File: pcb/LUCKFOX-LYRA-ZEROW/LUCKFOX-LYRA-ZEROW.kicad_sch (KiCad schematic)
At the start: 4 parts, among them U1 Luckfox_Lyra_Zero_W, U2 ME54BS12-nRF54L15, U3 ME54BS01-nRF54L15, U4 MCP2518FD-xQBB

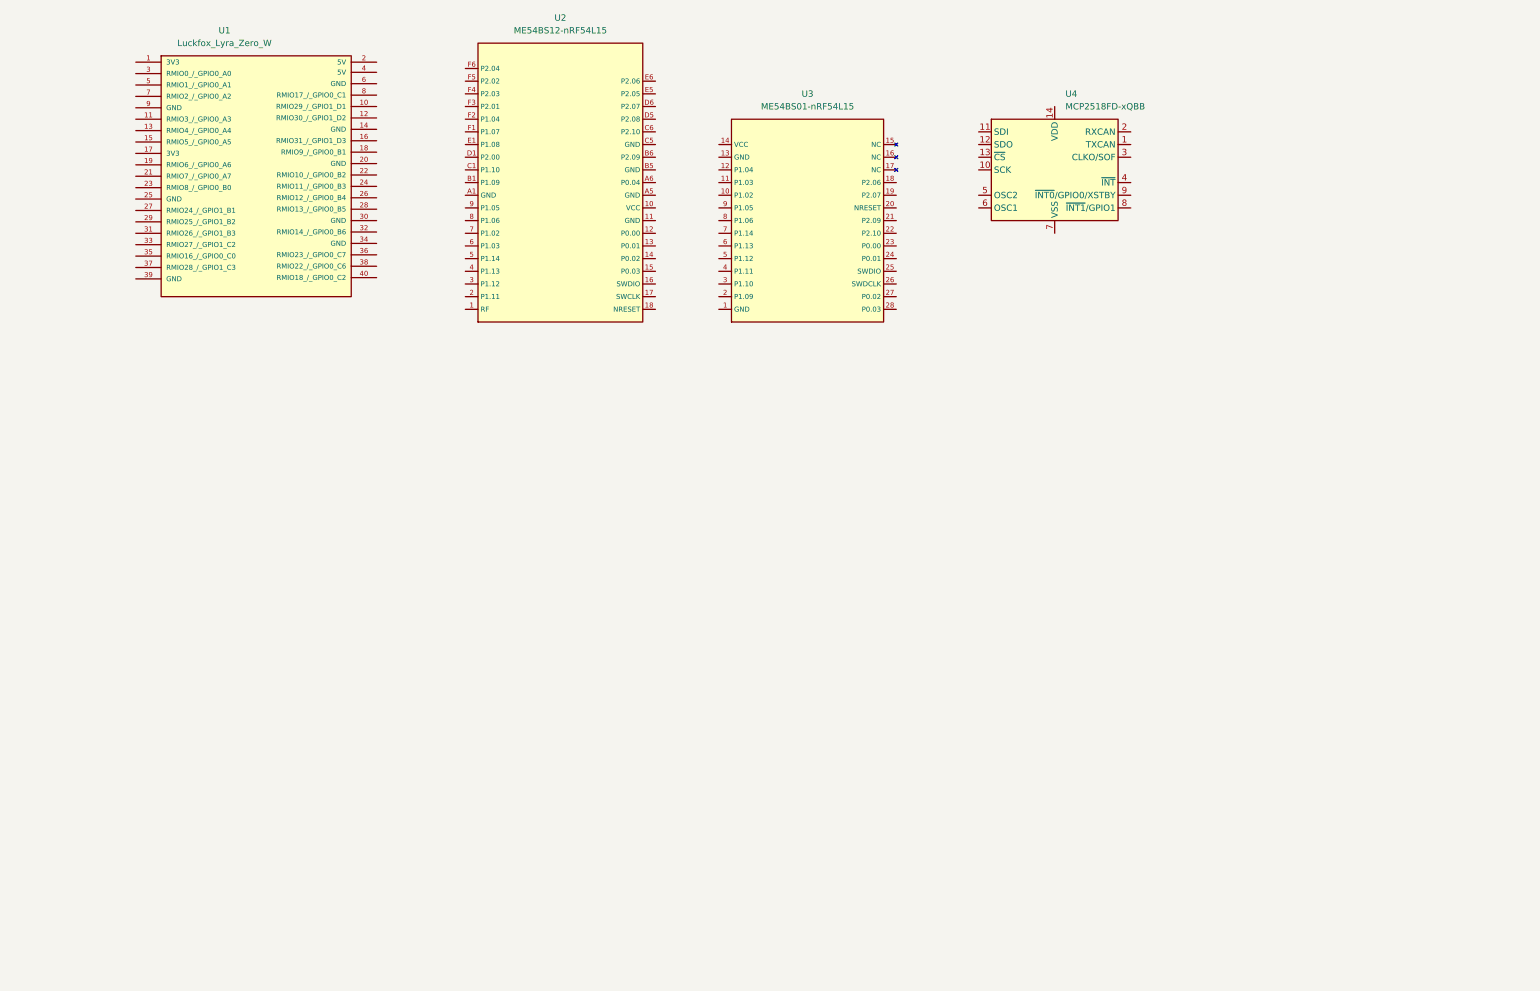
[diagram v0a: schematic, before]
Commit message: more pcb work
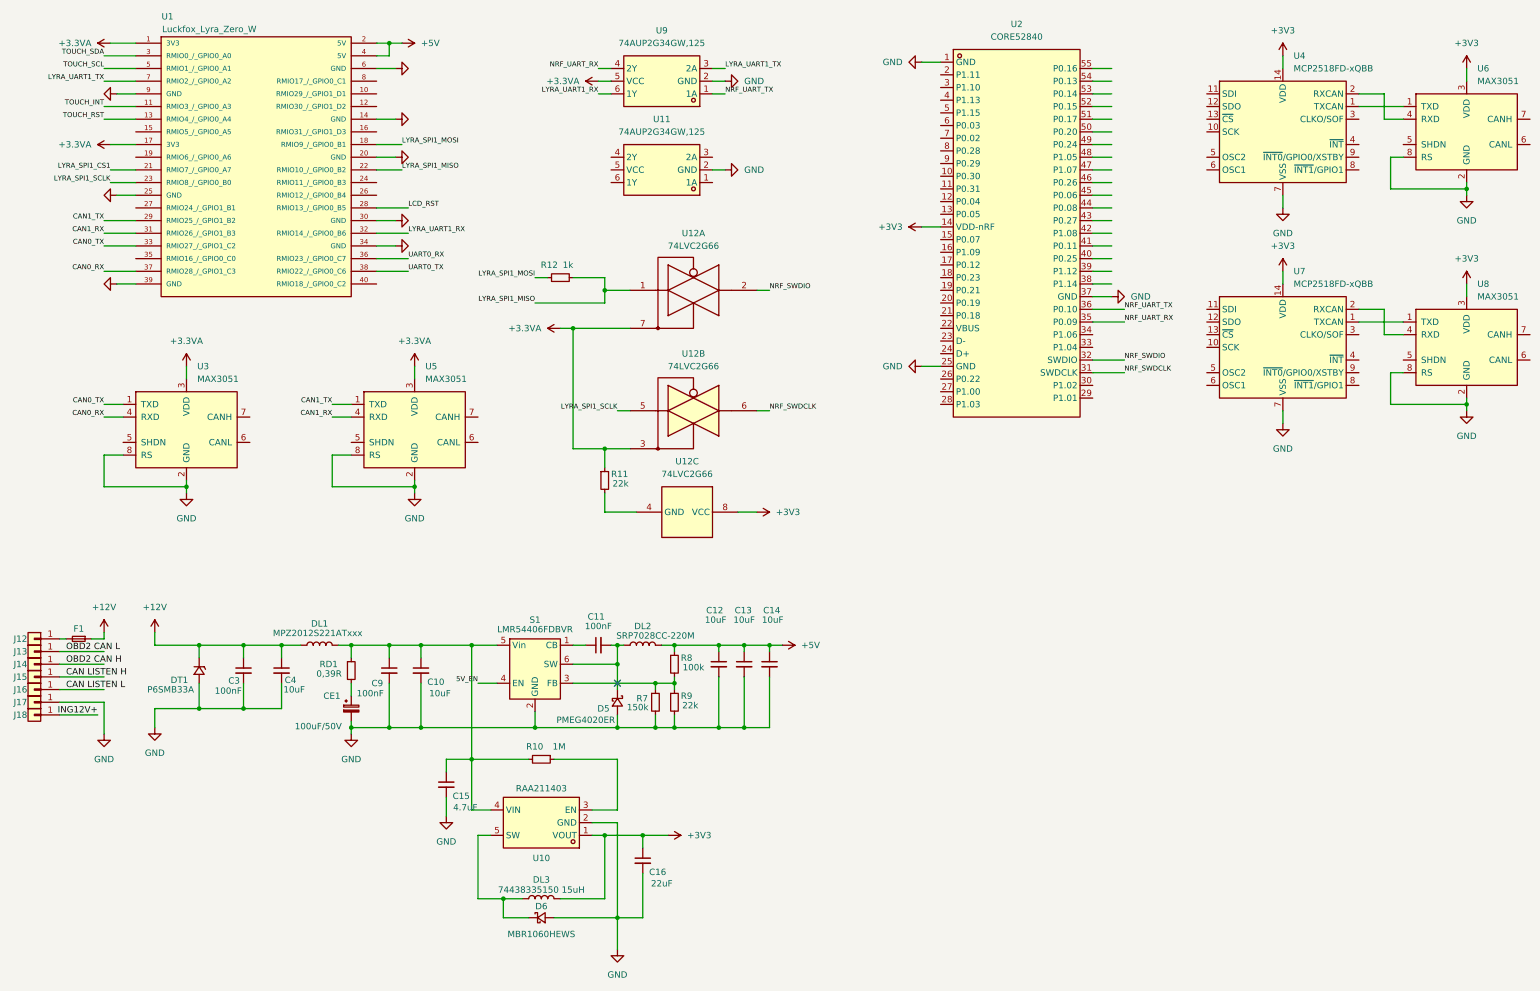
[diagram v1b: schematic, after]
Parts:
- removed U2: ME54BS12-nRF54L15, MinewSemi_nRF54:ME54BS12_nRF54L15, symbol MinewSemi_nRF54:ME54BS12_nRF54L15
- removed U3: ME54BS01-nRF54L15, MinewSemi_nRF54:ME54BS01_nRF54L15, symbol MinewSemi_nRF54:ME54BS01_nRF54L15
- added C10, C15, C4: 10uF/50V-X5R(X7R)_1206, ETH3:C_1206(3216), symbol ETH3:C_small_PG
- added C11, C3, C9: 100nF/50V-X7R_0805, ETH3:C_0805(2012), symbol ETH3:C_small_PG
- added C12, C13, C14: 10uF/16V(25V,35V,50V)-X5R(X7R)_1206, ETH3:C_1206(3216), symbol ETH3:C_small_PG
- added C16: 10uF/50V-X5R(X7R)_1206, symbol ETH3:C_small_PG
- added CE1: 100uF/50V EEUFR1H101, EEUFR1V101(100uF/35V), EEUF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, ETH3:CE_Radial_D8.0mm_P3.50mm, symbol ETH3:C_polarized_small
- added D5: PMEG4020ER, ETH3:SOD-123F_SOD123W_CFP3, symbol ETH3:D_Schott_small_PG
- added D6: PMEG4020ER, symbol ETH3:D_Schott_small_PG
- added DL1: MPZ2012S221ATxxx (MPZ2012S331ATxxx), (BLM21PG221S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, ETH3:R_0805(2012), symbol ETH3:L_small
- added DL2: SRP7028CC-220M (SRP7028A-220M), (SRP7028AA-220M),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, ETH3:L_BOURNS_SRP7028, symbol ETH3:L_small
- added DL3: SRP7028CC-220M (SRP7028A-220M), (SRP7028AA-220M),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, symbol ETH3:L_small
- added DT1: P6SMB33A, ETH3:D_SMB, symbol ETH3:D_Zen_PESD_small
- added F1: Fuse_Small, Fuse:Fuseholder_Littelfuse_Nano2_154x, symbol Device:Fuse_Small
- added J12, J13, J14, J15, J16, J17, J18: Conn_01x01, TestPoint:TestPoint_THTPad_1.0x1.0mm_Drill0.5mm, symbol Connector_Generic:Conn_01x01
- added R10, R7: (150k/1%_0805), ETH3:R_0805(2012), symbol ETH3:R_small_PG
- added R11, R12, R9: 22k/1%_0805, ETH3:R_0805(2012), symbol ETH3:R_small_PG
- added R8: 100k/1%_0805, ETH3:R_0805(2012), symbol ETH3:R_small_PG
- added RD1: 0,39R MMA02040C 3907J(G,F) (0,33R MMA02040C 3307J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, ETH3:R_MiniMELF-0204, symbol ETH3:R_small_PG
- added S1: LMR54406FDBVR (LMR54410FDBVR), (LMR54406DBVR), (L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, ETH3:SOT-23-6, symbol ETH3:LMR54406FDBVR
- added U10: RAA211403, RAA211403:SOT-23-5_L3.0-W1.7-P0.95-LS2.8-BL, symbol RAA211403:RAA2114034GP3#JA0
- added U11, U9: 74AUP2G34GW,125, Package_TO_SOT_SMD:SOT-363_SC-70-6_Handsoldering, symbol 74AUP2G34:74AUP2G34GW,125
- added U12: 74LVC2G66, RAA211403:SOT-23-5_L3.0-W1.7-P0.95-LS2.8-BL, symbol 74xGxx:74LVC2G66
- added U2: CORE52840, Core52840:BULETM-SMD_HOLYIOT-18010-NRF52840, symbol Core52840:CORE52840
- added U3, U5, U6, U8: MAX3051, Package_SO:SOIC-8_3.9x4.9mm_P1.27mm, symbol Interface_UART:MAX3051
- added U7: MCP2518FD-xQBB, Package_DFN_QFN:DFN-14-1EP_3x4.5mm_P0.65mm_EP1.65x4.25mm, symbol Interface_CAN_LIN:MCP2518FD-xQBB
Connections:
- net +3.3VA: now reaches U1.1 (3V3)
- net +3.3VA: now also U1.17 (3V3), R11.1, U12.3, U12.7, U3.3 (VDD), U5.3 (VDD), U9.5 (VCC)
- net TOUCH_INT: now reaches U1.11 (RMIO3_/_GPIO0_A3)
- net TOUCH_RST: now reaches U1.13 (RMIO4_/_GPIO0_A4)
- net GND: now reaches U1.14 (GND)
- net GND: now also U1.20 (GND), U1.25 (GND), U1.30 (GND), U1.34 (GND), U1.39 (GND), U1.6 (GND), U1.9 (GND), U4.15 (VSS), U4.7 (VSS), C10.2, C12.2, C13.2, C14.2, C15.2, C16.2, C3.2, C4.2, C9.2, CE1.2, D5.2 (A), D6.2 (A), DT1.2, J17.1 (Pin_1), R7.2, R9.2, S1.2 (GND), U10.2 (GND), U11.2 (GND), U2.1 (GND), U2.25 (GND), U2.37 (GND), U3.2 (GND), U3.8 (RS), U5.2 (GND), U5.8 (RS), U6.2 (GND), U6.8 (RS), U7.15 (VSS), U7.7 (VSS), U8.2 (GND), U8.8 (RS), U9.2 (GND)
- net LYRA_SPI1_MOSI: now reaches U1.18 (RMIO9_/_GPIO0_B1)
- net LYRA_SPI1_MOSI: now also R12.1
- net +5V: now reaches U1.2 (5V)
- net +5V: now also U1.4 (5V), C12.1, C13.1, C14.1, DL2.2, R8.1
- net LYRA_SPI1_CS1: now reaches U1.21 (RMIO7_/_GPIO0_A7)
- net LYRA_SPI1_MISO: now reaches U1.22 (RMIO10_/_GPIO0_B2)
- net LYRA_SPI1_MISO: now also R12.2, U12.1
- net LYRA_SPI1_SCLK: now reaches U1.23 (RMIO8_/_GPIO0_B0)
- net LYRA_SPI1_SCLK: now also U12.5
- net LCD_RST: now reaches U1.28 (RMIO13_/_GPIO0_B5)
- net CAN1_TX: now reaches U1.29 (RMIO25_/_GPIO1_B2)
- net CAN1_TX: now also U5.1 (TXD)
- net TOUCH_SDA: now reaches U1.3 (RMIO0_/_GPIO0_A0)
- net CAN1_RX: now reaches U1.31 (RMIO26_/_GPIO1_B3)
- net CAN1_RX: now also U5.4 (RXD)
- net LYRA_UART1_RX: now reaches U1.32 (RMIO14_/_GPIO0_B6)
- net LYRA_UART1_RX: now also U9.6 (1Y)
- net CAN0_TX: now reaches U1.33 (RMIO27_/_GPIO1_C2)
- net CAN0_TX: now also U3.1 (TXD)
- net UART0_RX: now reaches U1.36 (RMIO23_/_GPIO0_C7)
- net CAN0_RX: now reaches U1.37 (RMIO28_/_GPIO1_C3)
- net CAN0_RX: now also U3.4 (RXD)
- net UART0_TX: now reaches U1.38 (RMIO22_/_GPIO0_C6)
- net TOUCH_SCL: now reaches U1.5 (RMIO1_/_GPIO0_A1)
- net LYRA_UART1_TX: now reaches U1.7 (RMIO2_/_GPIO0_A2)
- net LYRA_UART1_TX: now also U9.3 (2A)
- net at U4.1 (TXCAN): now also U6.1 (TXD)
- net +3V3: now reaches U4.14 (VDD)
- net +3V3: now also C16.1, DL3.2, U10.1 (VOUT), U12.8 (VCC), U2.14 (VDD-nRF), U6.3 (VDD), U7.14 (VDD), U8.3 (VDD)
- net at U4.2 (RXCAN): now also U6.4 (RXD)
- new net: C10.1, C15.1, C9.1, DL1.2, R10.2, RD1.1, S1.5 (Vin), U10.4 (VIN)
- new net: C11.2, D5.1 (K), DL2.1, S1.6 (SW)
- new net: F1.2, J12.1 (Pin_1)
- new net: D6.1 (K), DL3.1, U10.5 (SW)
- new net: R10.1, U10.3 (EN)
- new net: R7.1, R8.2, R9.1, S1.3 (FB)
- new net: C11.1, S1.1 (CB)
- new net: CE1.1, RD1.2
- new net: R11.2, U12.4 (GND)
- new net: U7.1 (TXCAN), U8.1 (TXD)
- new net: U7.2 (RXCAN), U8.4 (RXD)
- new net +12V: C3.1, C4.1, DL1.1, DT1.1, F1.1
- new net 5V_EN: S1.4 (EN)
- new net CAN LISTEN H: J15.1 (Pin_1)
- new net CAN LISTEN L: J16.1 (Pin_1)
- new net ING12V+: J18.1 (Pin_1)
- new net NRF_SWDCLK: U12.6, U2.31 (SWDCLK)
- new net NRF_SWDIO: U12.2, U2.32 (SWDIO)
- new net NRF_UART_RX: U2.35 (P0.09), U9.4 (2Y)
- new net NRF_UART_TX: U2.36 (P0.10), U9.1 (1A)
- new net OBD2 CAN H: J14.1 (Pin_1)
- new net OBD2 CAN L: J13.1 (Pin_1)
- no-connect marks 0 -> 1
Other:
- moved on the sheet: U1, U4
